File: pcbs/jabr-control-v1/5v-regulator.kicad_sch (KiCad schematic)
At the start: 0 parts

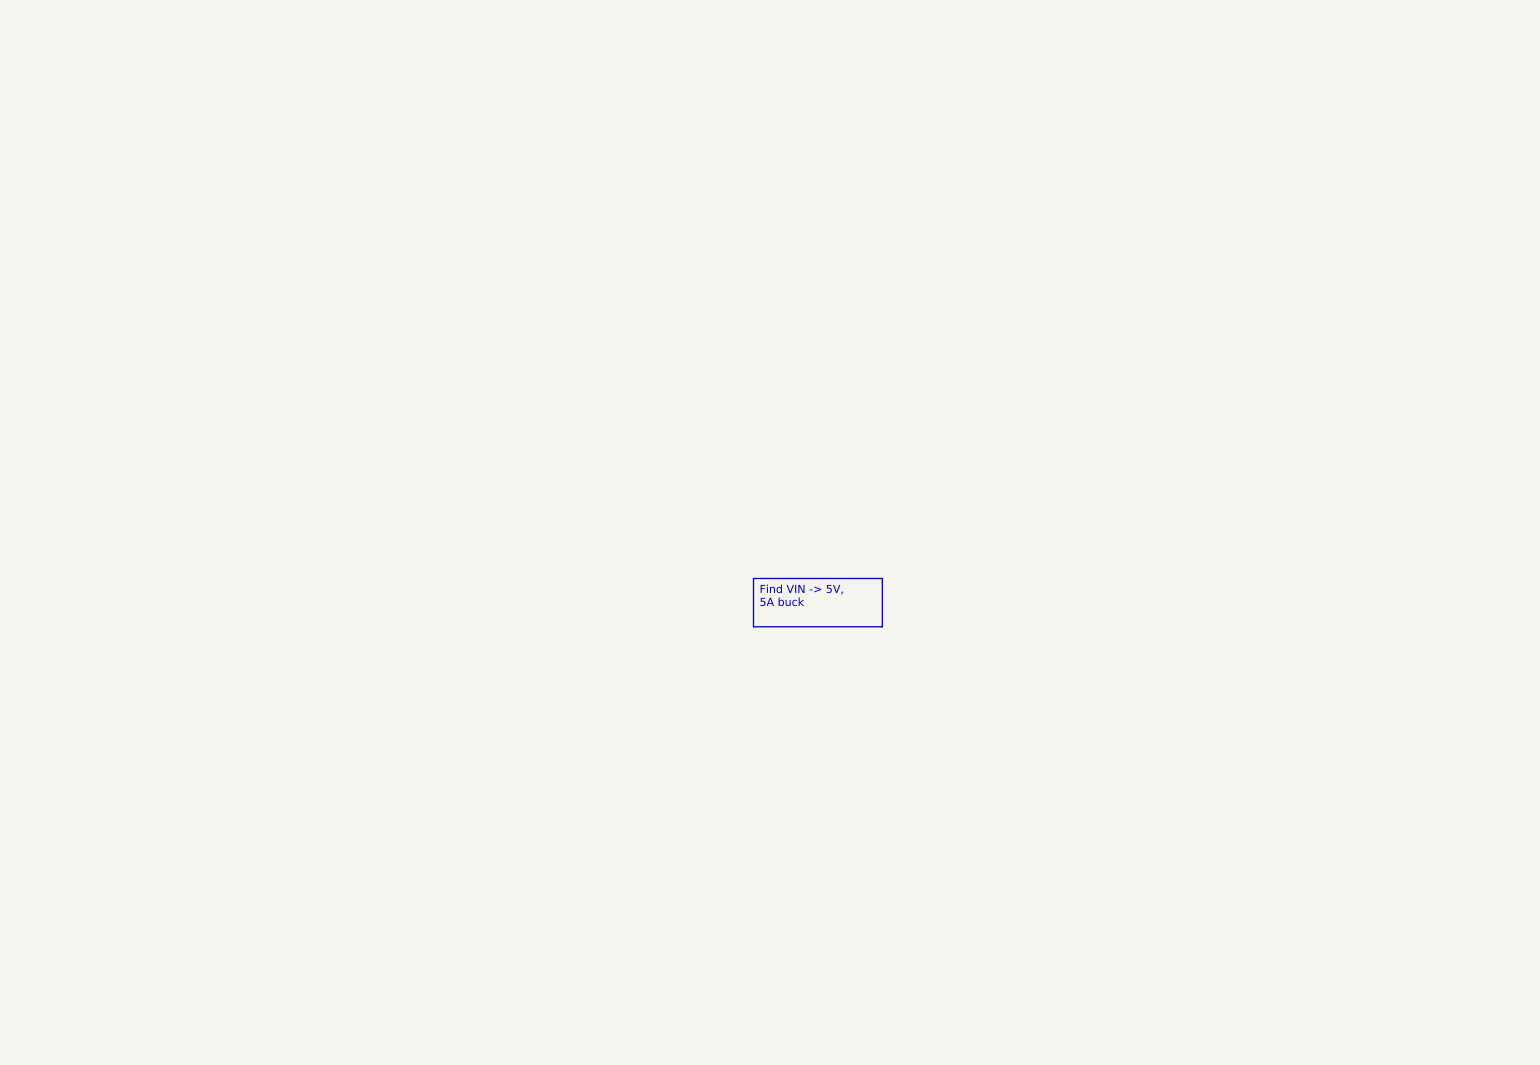
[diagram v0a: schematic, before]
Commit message: Worked on power and other areas of the schematic
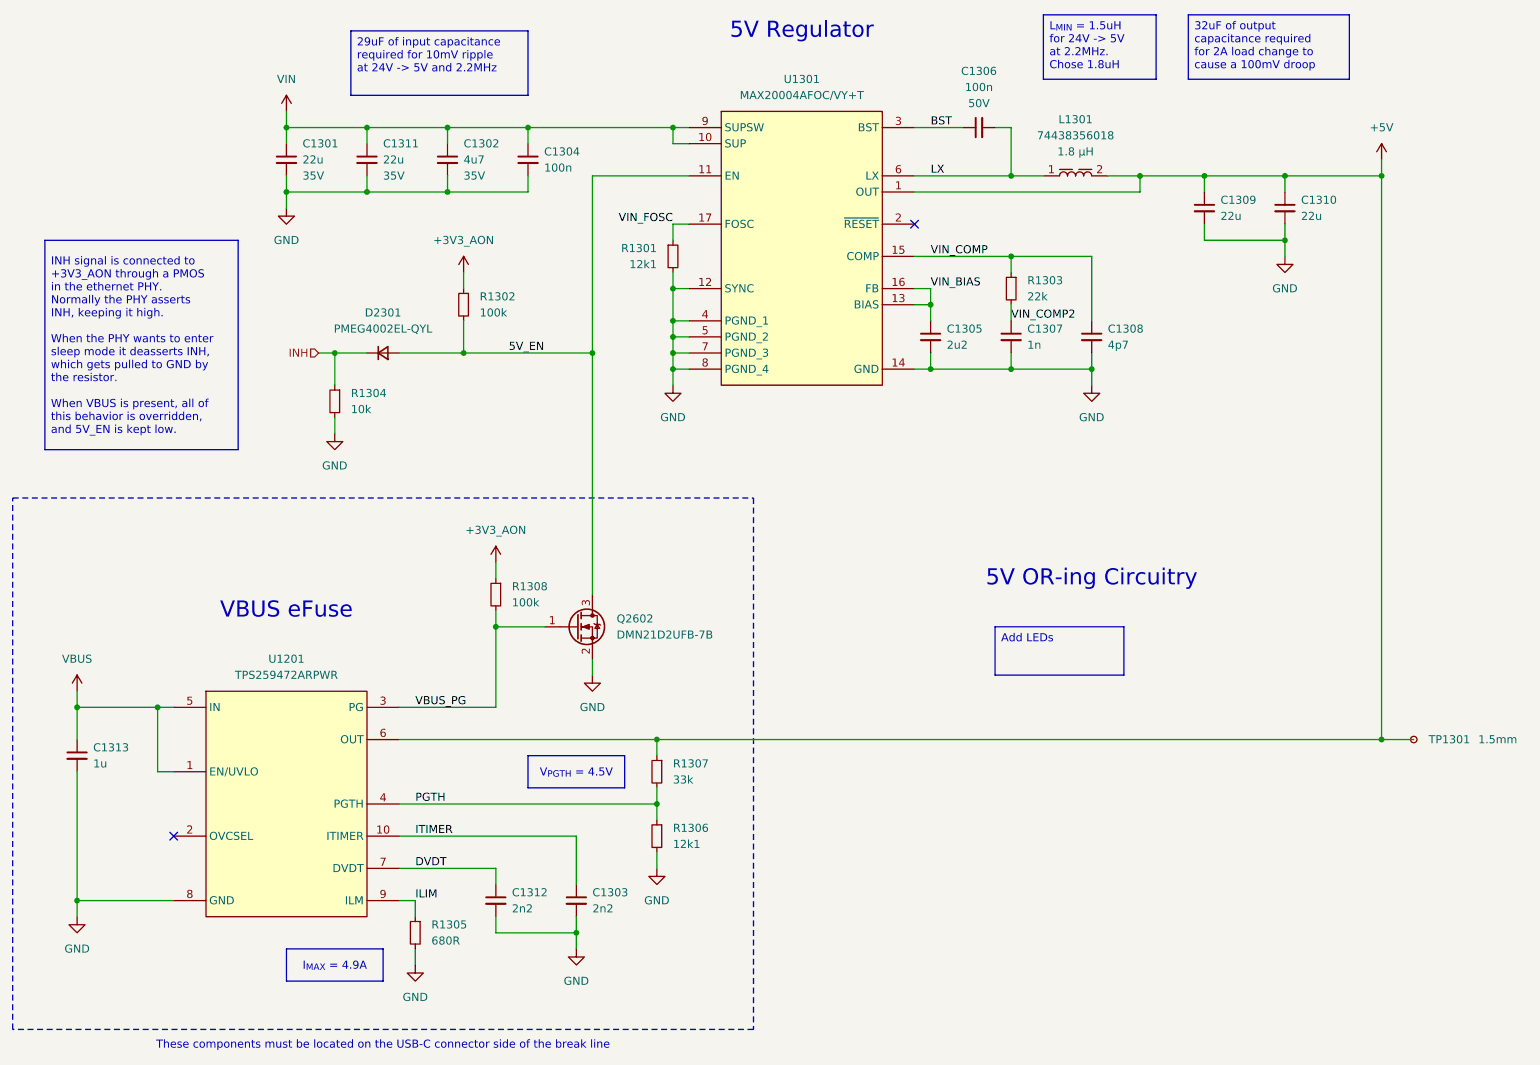
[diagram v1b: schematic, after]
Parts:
- added C1301, C1309, C1310, C1311: 22u, Capacitor_SMD:C_0805_2012Metric, symbol Device:C_Small
- added C1302: 4u7, Capacitor_SMD:C_0805_2012Metric, symbol Device:C_Small
- added C1303, C1312: 2n2, project_footprints:C_0402, symbol Device:C_Small
- added C1304, C1306: 100n, project_footprints:C_0402, symbol Device:C_Small
- added C1305: 2u2, project_footprints:C_0402, symbol Device:C_Small
- added C1307: 1n, project_footprints:C_0402, symbol Device:C_Small
- added C1308: 4p7, project_footprints:C_0402, symbol Device:C_Small
- added C1313: 1u, project_footprints:C_0402, symbol Device:C_Small
- added D2301: PMEG4002EL-QYL, project_footprints:PMEG4002EL-QYL, symbol DIODE:PMEG4002EL-QYL
- added L1301: 74438356018, Inductor_SMD_Wurth:L_Wurth_WE-MAPI-4020, symbol PWR-IND:4020_74438356018
- added Q2602: DMN21D2UFB-7B, project_footprints:DMN21D2UFB7B, symbol MOSFET:DMN21D2UFB-7B
- added R1301, R1306: 12k1, project_footprints:R_0402, symbol Device:R_Small
- added R1302, R1308: 100k, project_footprints:R_0402, symbol Device:R_Small
- added R1303: 22k, project_footprints:R_0402, symbol Device:R_Small
- added R1304: 10k, project_footprints:R_0402, symbol Device:R_Small
- added R1305: 680R, project_footprints:R_0402, symbol Device:R_Small
- added R1307: 33k, project_footprints:R_0402, symbol Device:R_Small
- added TP1301: 1.5mm, TestPoint:TestPoint_Pad_D1.5mm, symbol Connector:TestPoint_Small
- added U1201: TPS259472ARPWR, project_footprints:TPS259472ARPWR, symbol PWR-SWCH:TPS259472ARPWR
- added U1301: MAX20004AFOC/VY+T, project_footprints:MAX20004AFOC_VY+, symbol MAX-SMPS:MAX20004AFOA_VY+T
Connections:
- new net +3V3_AON: R1302.1, R1308.1
- new net +5V: C1309.1, C1310.1, L1301.2, R1307.1, TP1301.1, U1201.6 (OUT), U1301.1 (OUT)
- new net 5V_EN: D2301.2 (A), Q2602.3 (D), R1302.2, U1301.11 (EN)
- new net BST: C1306.1, U1301.3 (BST)
- new net DVDT: C1312.1, U1201.14 (DVDT), U1201.7 (DVDT)
- new net GND: C1301.2, C1302.2, C1303.2, C1304.2, C1305.2, C1307.2, C1308.2, C1309.2, C1310.2, C1311.2, C1312.2, C1313.2, Q2602.2 (S), R1301.2, R1304.2, R1305.2, R1306.2, U1201.8 (GND), U1301.12 (SYNC), U1301.14 (GND), U1301.4 (PGND_1), U1301.5 (PGND_2), U1301.7 (PGND_3), U1301.8 (PGND_4)
- new net ILIM: R1305.1, U1201.9 (ILM)
- new net INH: D2301.1 (K), R1304.1
- new net ITIMER: C1303.1, U1201.10 (ITIMER), U1201.11 (ITIMER)
- new net LX: C1306.2, L1301.1, U1301.6 (LX)
- new net PGTH: R1306.1, R1307.2, U1201.13 (PGTH), U1201.4 (PGTH)
- new net VBUS: C1313.1, U1201.1 (EN/UVLO), U1201.12 (EN/UVLO), U1201.5 (IN)
- new net VBUS_PG: Q2602.1 (G), R1308.2, U1201.3 (PG)
- new net VIN: C1301.1, C1302.1, C1304.1, C1311.1, U1301.10 (SUP), U1301.9 (SUPSW)
- new net VIN_BIAS: C1305.1, U1301.13 (BIAS), U1301.16 (FB)
- new net VIN_COMP: C1308.1, R1303.1, U1301.15 (COMP)
- new net VIN_COMP2: C1307.1, R1303.2
- new net VIN_FOSC: R1301.1, U1301.17 (FOSC)
- no-connect marks 0 -> 2
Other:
- note added: "5V OR-ing Circuitry"
- note added: "5V Regulator"
- note added: "These components must be located on the USB-C connector side of the break line"
- note added: "VBUS eFuse"
